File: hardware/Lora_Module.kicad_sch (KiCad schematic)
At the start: 1 part, among them U7 RFM95W-868S2

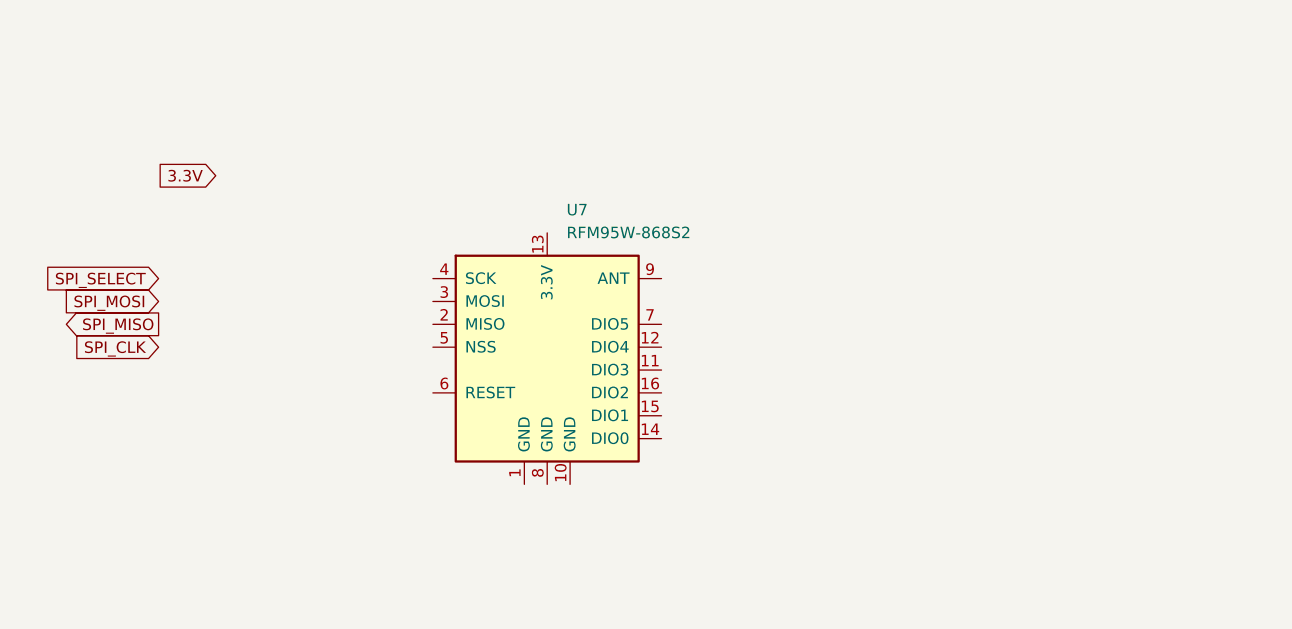
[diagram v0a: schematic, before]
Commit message: Module Lora
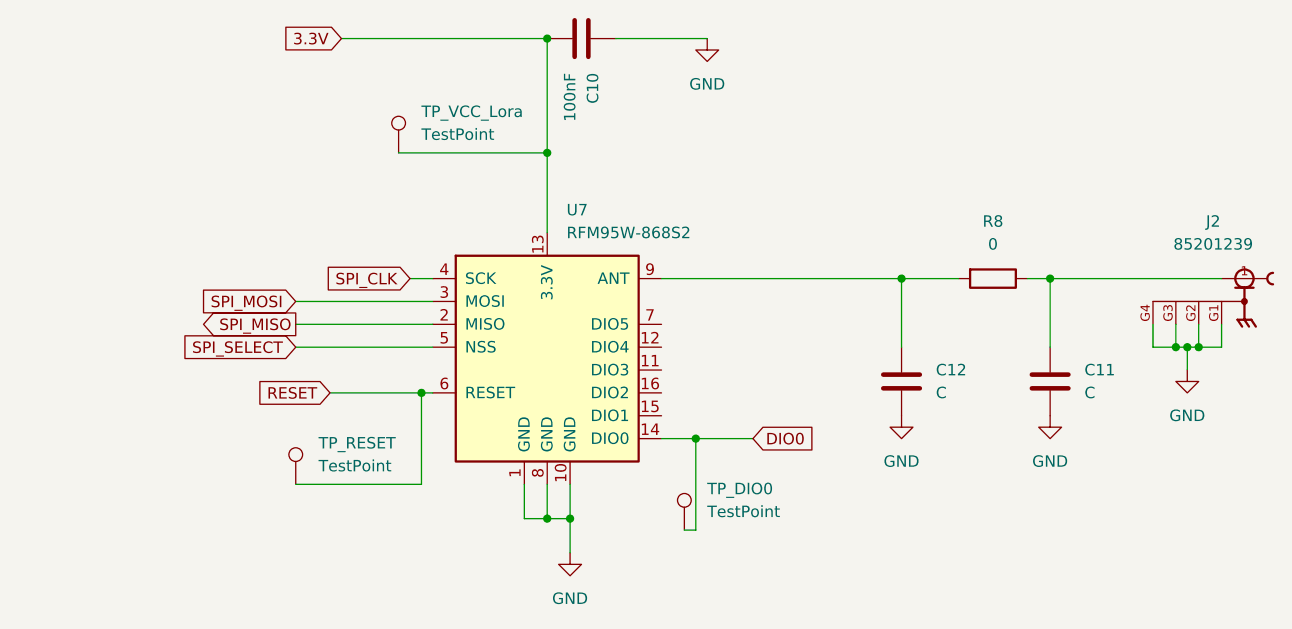
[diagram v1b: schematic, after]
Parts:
- added C10: 100nF, Capacitor_SMD:C_0201_0603Metric, symbol Device:C
- added C11, C12: C, Capacitor_SMD:C_0805_2012Metric_Pad1.18x1.45mm_HandSolder, symbol Device:C
- added J2: 85201239, SMA-85201239:HUBER_SUHNER_85201239, symbol SMA-85201239:85201239
- added R8: 0, Resistor_SMD:R_0805_2012Metric_Pad1.20x1.40mm_HandSolder, symbol Device:R
- added TP_DIO0, TP_RESET, TP_VCC_Lora: TestPoint, TestPoint:TestPoint_Pad_D2.0mm, symbol Connector:TestPoint
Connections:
- net 3.3V: now also U7.13 (3.3V), C10.2, TP_VCC_Lora.1
- net SPI_CLK: now also U7.4 (SCK)
- net SPI_MISO: now also U7.2 (MISO)
- net SPI_MOSI: now also U7.3 (MOSI)
- net SPI_SELECT: now also U7.5 (NSS)
- net GND: now reaches U7.1 (GND)
- net GND: now also U7.10 (GND), U7.8 (GND), C10.1, C11.2, C12.2, J2.G1, J2.G2, J2.G3, J2.G4
- net DIO0: now reaches U7.14 (DIO0)
- net DIO0: now also TP_DIO0.1
- net RESET: now reaches U7.6 (RESET)
- net RESET: now also TP_RESET.1
- net at U7.9 (ANT): now also C12.1, R8.2
- new net: C11.1, J2.1, R8.1
